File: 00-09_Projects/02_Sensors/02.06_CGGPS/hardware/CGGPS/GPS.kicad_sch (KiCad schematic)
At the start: 7 parts, among them J3 Conn_Coaxial, U2 ZED-F9P-02B

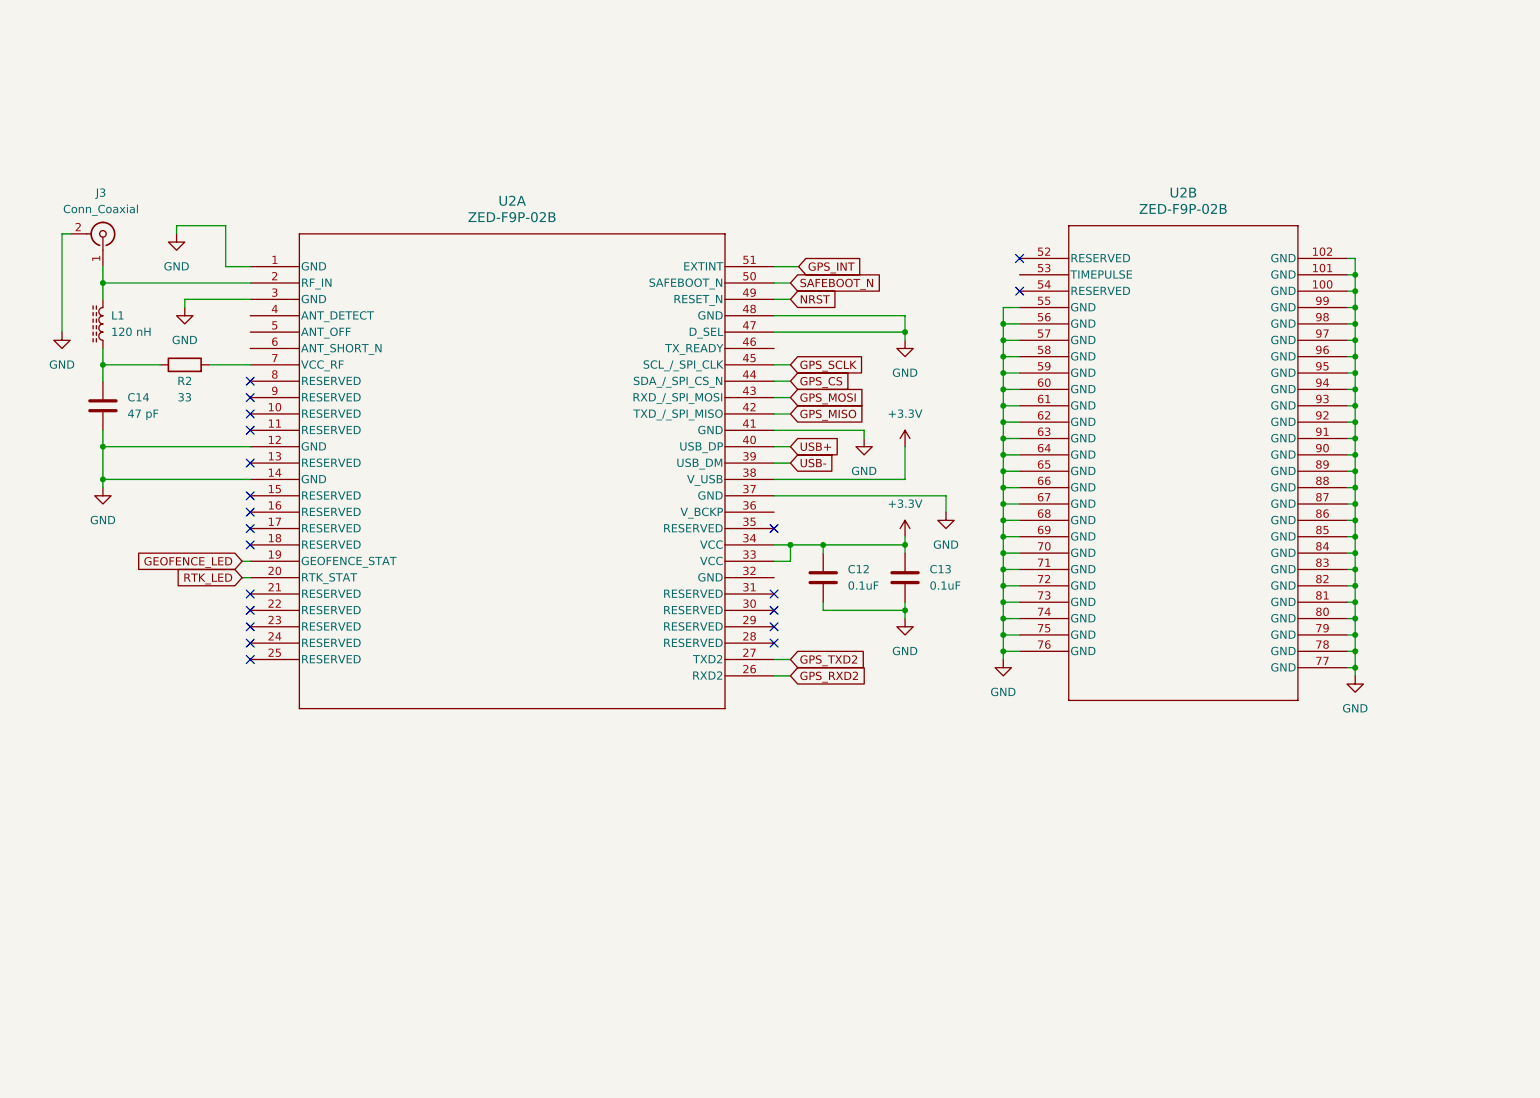
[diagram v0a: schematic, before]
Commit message: wip
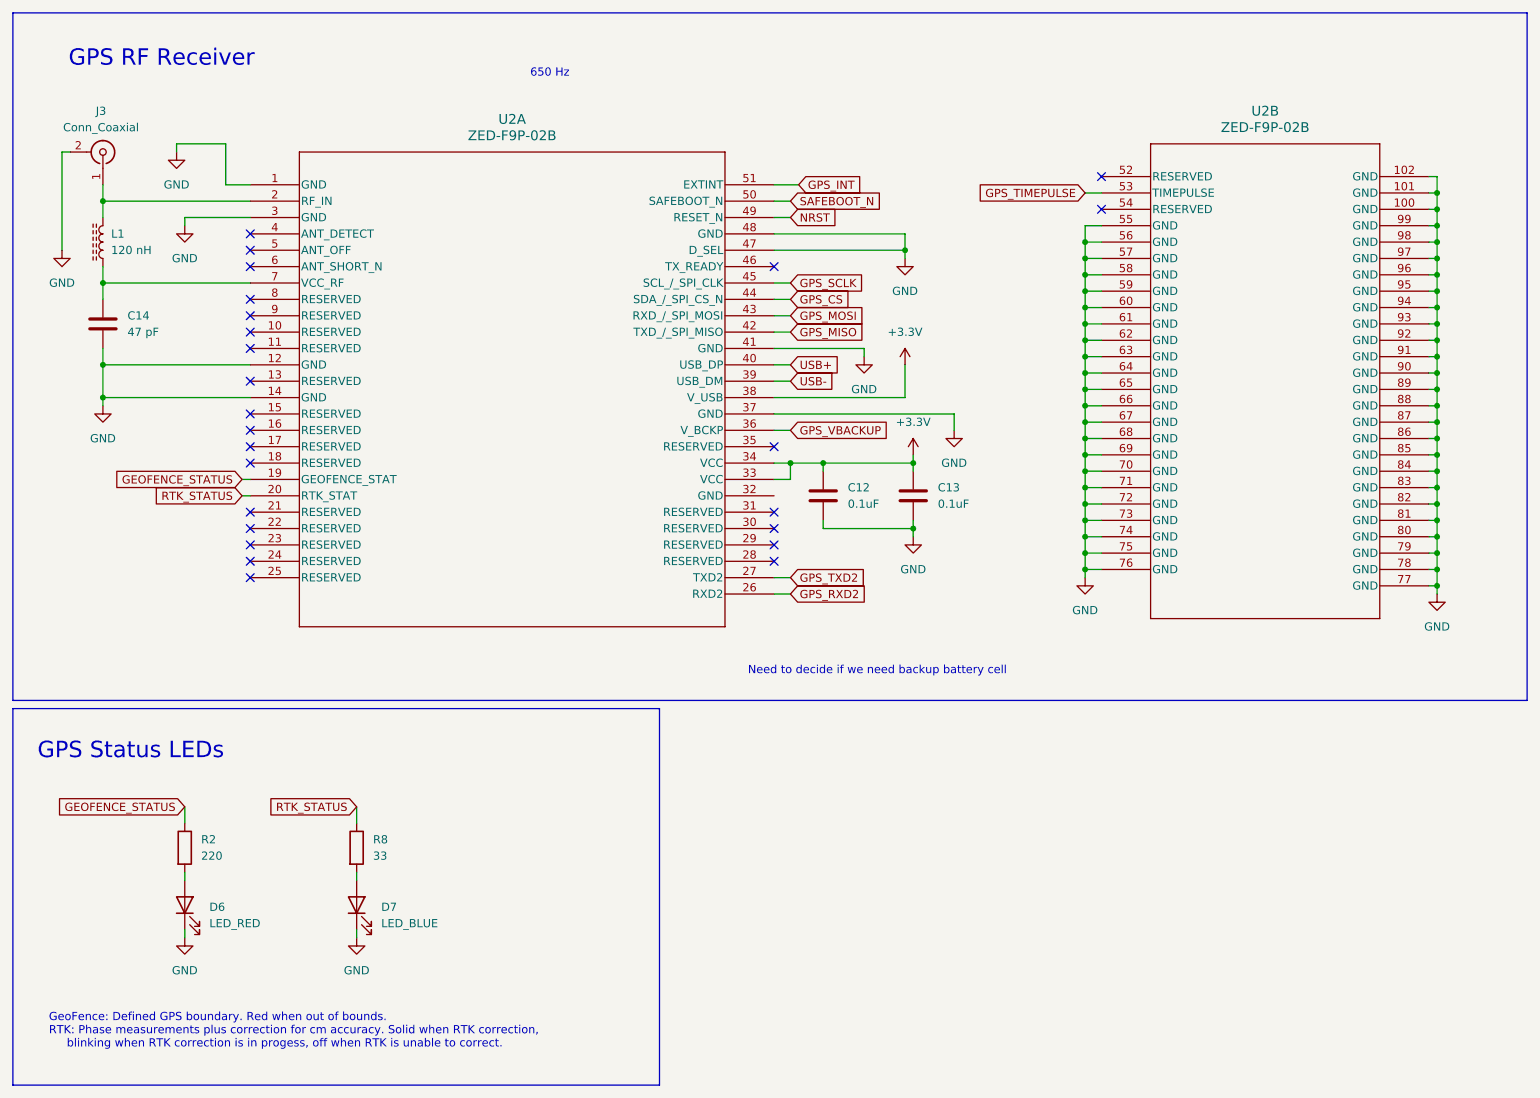
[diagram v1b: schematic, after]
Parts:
- added D6: LED_RED, symbol Device:LED
- added D7: LED_BLUE, symbol Device:LED
- added R8: 33, symbol Device:R
- R2: value 33 -> 220
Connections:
- net GND: now also D6.1 (K), D7.1 (K)
- net GPS_TIMEPULSE: now reaches U2.53 (TIMEPULSE)
- net at C14.1, L1.1: now also U2.7 (VCC_RF); no longer R2.1
- net at R2.2: now also D6.2 (A); no longer U2.7 (VCC_RF)
- net GPS_VBACKUP: now reaches U2.36 (V_BCKP)
- net GEOFENCE_LED renamed GEOFENCE_STATUS
- net GEOFENCE_STATUS: now also R2.1
- net RTK_LED renamed RTK_STATUS
- net RTK_STATUS: now also R8.1
- new net: D7.2 (A), R8.2
- no-connect marks 21 -> 25
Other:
- note added: "650 Hz"
- note added: "GPS RF Receiver"
- note added: "GPS Status LEDs"
- note added: "GeoFence: Defined GPS boundary. Red when out of bounds. RTK: Phase measurements plus correction for cm accuracy. Solid when RTK correction, blinking when RTK correction is in progess, off when RTK is unable to correct."
- note added: "Need to decide if we need backup battery cell"
- moved on the sheet: C12, C13, C14, J3, L1, U2A, U2B
